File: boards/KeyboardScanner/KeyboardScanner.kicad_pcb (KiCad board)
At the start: 2 copper layers, 150 x 100 mm, 36 parts, among them J1 Keyboard1, J2 Keyboard1, J3 Encoder, J4 Select, U1 74LS151, U10 74LS151, U11 TBD62783A, U2 74LS151, U3 74LS151, U4 74LS151, U6 74LS151, U7 74LS151, U8 4069, U9 74LS151

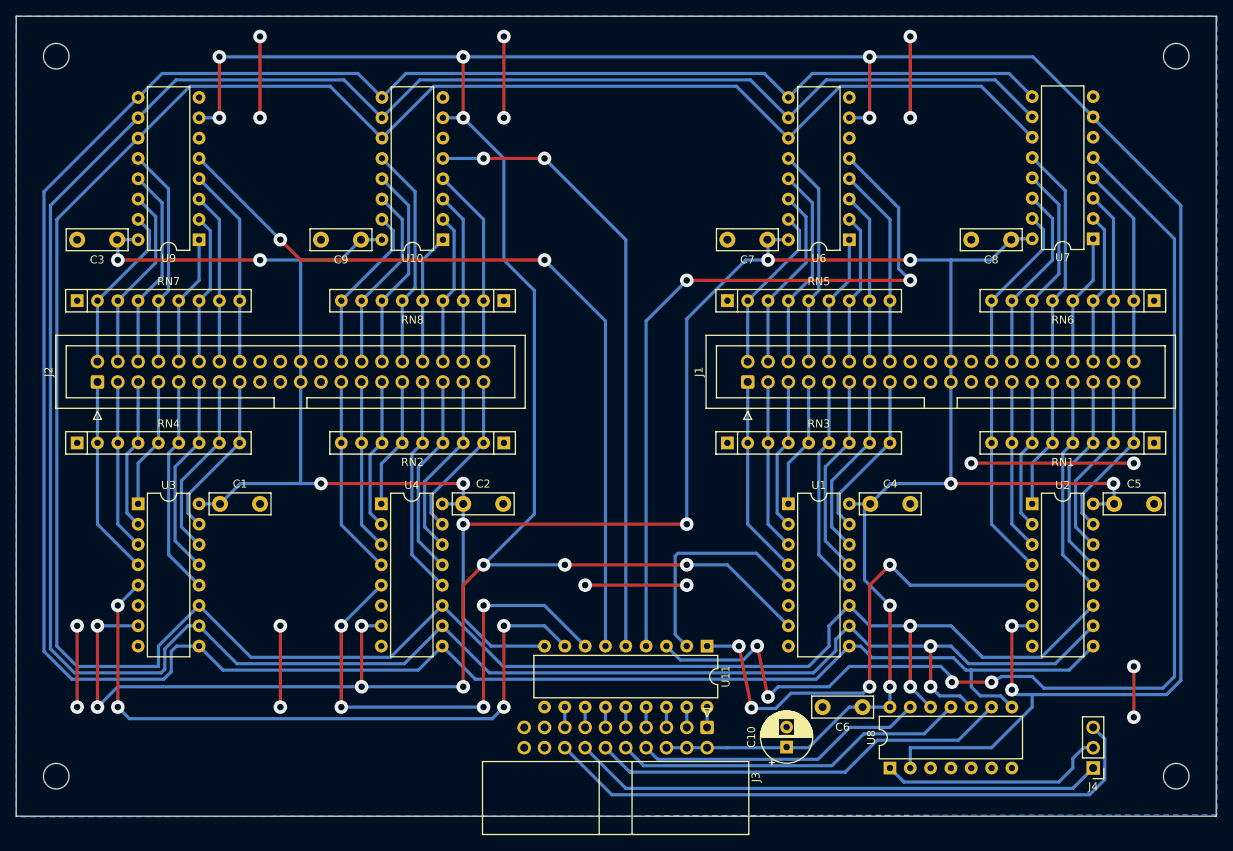
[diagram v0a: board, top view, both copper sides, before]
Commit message: Reverting to using 2803A inverted open collector for Keyboard Scanner, fixed layout
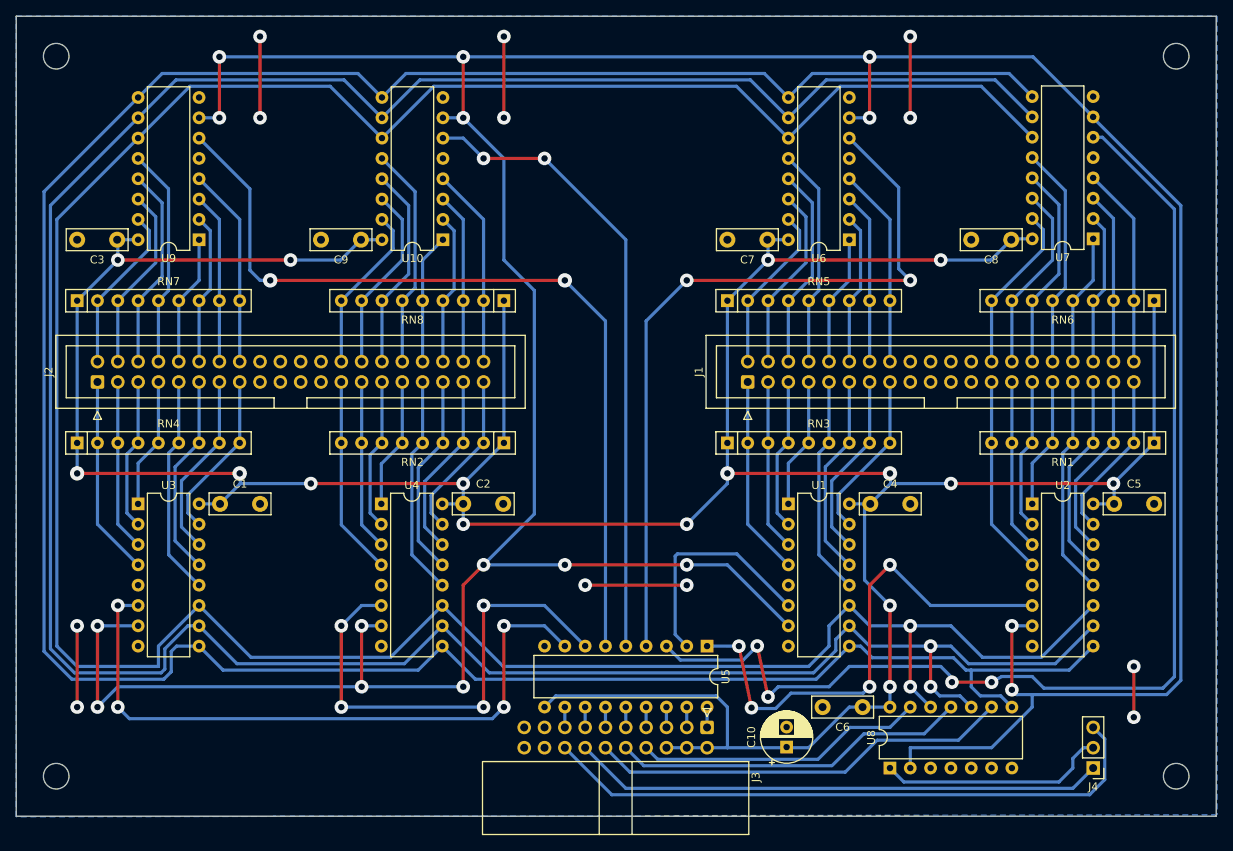
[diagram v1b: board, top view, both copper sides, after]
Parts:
- removed U11: TBD62783A, Package_DIP:DIP-18_W7.62mm
- added U5: ULN2803A, Package_DIP:DIP-18_W7.62mm, F.Cu at (162.6, 119.4)
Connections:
- J1 pad 21: +5V -> GND
- J1 pad 22: +5V -> GND
- J2 pad 21: +5V -> GND
- J2 pad 22: +5V -> GND
- RN1 pad 1: GND -> +5V
- RN2 pad 1: GND -> +5V
- RN3 pad 1: GND -> +5V
- RN4 pad 1: GND -> +5V
- RN5 pad 1: GND -> +5V
- RN6 pad 1: GND -> +5V
- RN7 pad 1: GND -> +5V
- RN8 pad 1: GND -> +5V
- U1 pad 5: O1 -> unconnected-(U1-Z-Pad5)
- U1 pad 6: unconnected-(U1-~{Z}-Pad6) -> O1
- U10 pad 5: O8 -> unconnected-(U10-Z-Pad5)
- U10 pad 6: unconnected-(U10-~{Z}-Pad6) -> O8
- U2 pad 5: O2 -> unconnected-(U2-Z-Pad5)
- U2 pad 6: unconnected-(U2-~{Z}-Pad6) -> O2
- U3 pad 5: O3 -> unconnected-(U3-Z-Pad5)
- U3 pad 6: unconnected-(U3-~{Z}-Pad6) -> O3
- U4 pad 5: O4 -> unconnected-(U4-Z-Pad5)
- U4 pad 6: unconnected-(U4-~{Z}-Pad6) -> O4
- U6 pad 5: O5 -> unconnected-(U6-Z-Pad5)
- U6 pad 6: unconnected-(U6-~{Z}-Pad6) -> O5
- U7 pad 5: O6 -> unconnected-(U7-Z-Pad5)
- U7 pad 6: unconnected-(U7-~{Z}-Pad6) -> O6
- U9 pad 5: O7 -> unconnected-(U9-Z-Pad5)
- U9 pad 6: unconnected-(U9-~{Z}-Pad6) -> O7
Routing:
- net +5V: track 362.4 -> 432.6 mm, vias 12 -> 16
- net GND: track 90.2 -> 59.7 mm, vias 16 -> 12
- net O7: track 99.9 -> 106.9 mm
- net O6: track 143.3 -> 146.5 mm
- net O5: track 93.7 -> 96.2 mm
- net O8: track 77.9 -> 78.9 mm
- net O2: track 62.9 -> 63.9 mm
- net O3: track 84.6 -> 83.5 mm
- net O4: track 62.6 -> 61.6 mm
- net O1: track 27.8 -> 28.8 mm

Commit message: Revert "Reverting to using 2803A inverted open collector for Keyboard Scanner, fixed layout"
This reverts commit 7b46a6886eac97662925cbadd02de0ff96663bd2.
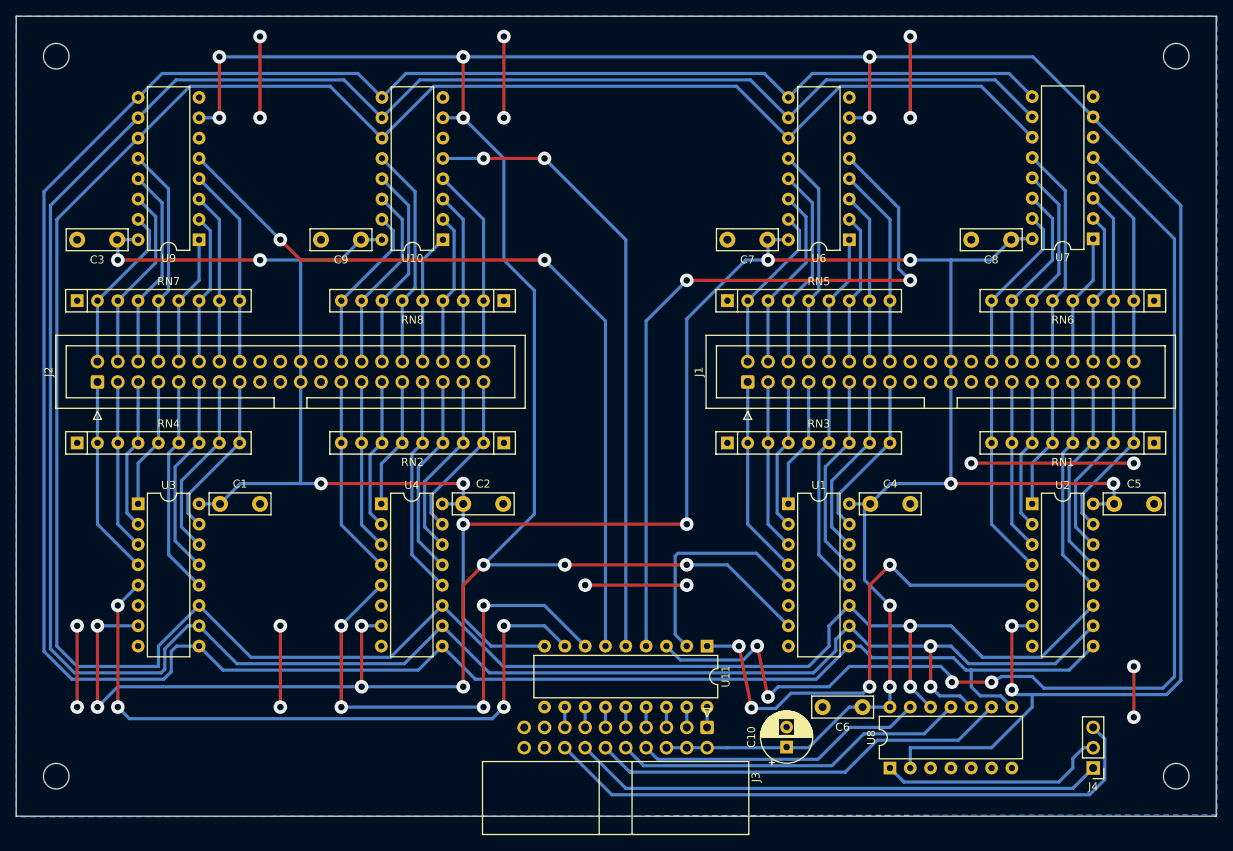
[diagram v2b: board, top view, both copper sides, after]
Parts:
- removed U5: ULN2803A, Package_DIP:DIP-18_W7.62mm
- added U11: TBD62783A, Package_DIP:DIP-18_W7.62mm, F.Cu at (162.6, 119.4)
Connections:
- J1 pad 21: GND -> +5V
- J1 pad 22: GND -> +5V
- J2 pad 21: GND -> +5V
- J2 pad 22: GND -> +5V
- RN1 pad 1: +5V -> GND
- RN2 pad 1: +5V -> GND
- RN3 pad 1: +5V -> GND
- RN4 pad 1: +5V -> GND
- RN5 pad 1: +5V -> GND
- RN6 pad 1: +5V -> GND
- RN7 pad 1: +5V -> GND
- RN8 pad 1: +5V -> GND
- U1 pad 5: unconnected-(U1-Z-Pad5) -> O1
- U1 pad 6: O1 -> unconnected-(U1-~{Z}-Pad6)
- U10 pad 5: unconnected-(U10-Z-Pad5) -> O8
- U10 pad 6: O8 -> unconnected-(U10-~{Z}-Pad6)
- U2 pad 5: unconnected-(U2-Z-Pad5) -> O2
- U2 pad 6: O2 -> unconnected-(U2-~{Z}-Pad6)
- U3 pad 5: unconnected-(U3-Z-Pad5) -> O3
- U3 pad 6: O3 -> unconnected-(U3-~{Z}-Pad6)
- U4 pad 5: unconnected-(U4-Z-Pad5) -> O4
- U4 pad 6: O4 -> unconnected-(U4-~{Z}-Pad6)
- U6 pad 5: unconnected-(U6-Z-Pad5) -> O5
- U6 pad 6: O5 -> unconnected-(U6-~{Z}-Pad6)
- U7 pad 5: unconnected-(U7-Z-Pad5) -> O6
- U7 pad 6: O6 -> unconnected-(U7-~{Z}-Pad6)
- U9 pad 5: unconnected-(U9-Z-Pad5) -> O7
- U9 pad 6: O7 -> unconnected-(U9-~{Z}-Pad6)
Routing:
- net +5V: track 432.6 -> 362.4 mm, vias 16 -> 12
- net GND: track 59.7 -> 90.2 mm, vias 12 -> 16
- net O7: track 106.9 -> 99.9 mm
- net O6: track 146.5 -> 143.3 mm
- net O5: track 96.2 -> 93.7 mm
- net O8: track 78.9 -> 77.9 mm
- net O2: track 63.9 -> 62.9 mm
- net O3: track 83.5 -> 84.6 mm
- net O4: track 61.6 -> 62.6 mm
- net O1: track 28.8 -> 27.8 mm
